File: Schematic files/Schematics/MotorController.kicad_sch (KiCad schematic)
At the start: 5 parts, among them M1 Z-Axis Stepper Motor

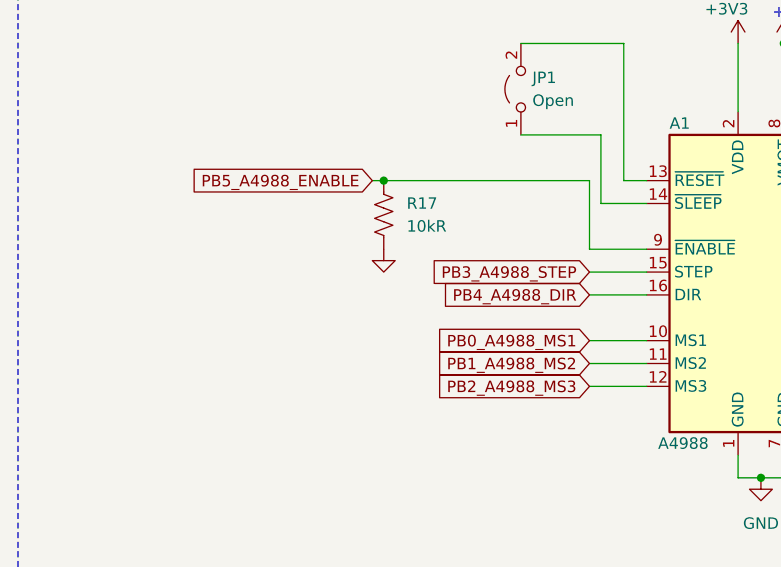
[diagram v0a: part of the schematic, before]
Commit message: pcb
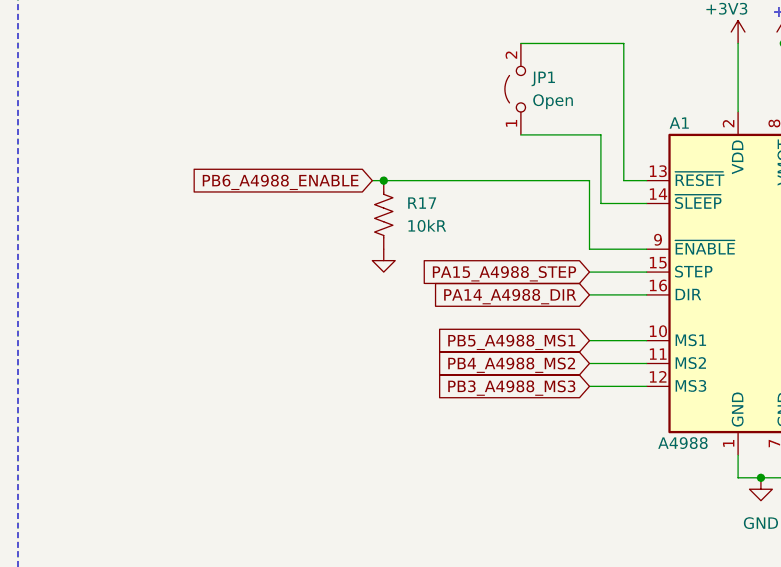
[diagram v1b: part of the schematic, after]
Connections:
- net PB0_A4988_MS1 renamed PB5_A4988_MS1
- net PB1_A4988_MS2 renamed PB4_A4988_MS2
- net PB2_A4988_MS3 renamed PB3_A4988_MS3
- net PB3_A4988_STEP renamed PA15_A4988_STEP
- net PB4_A4988_DIR renamed PA14_A4988_DIR
- net PB5_A4988_ENABLE renamed PB6_A4988_ENABLE
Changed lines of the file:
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@@
     (effects (font (size 1.27 1.27)) (justify left bottom))
   )
-  (global_label "PB1_A4988_MS2" (shape input) (at 115.57 73.66 180) (fields_autoplaced)
+  (global_label "PB4_A4988_MS2" (shape input) (at 115.57 73.66 180) (fields_autoplaced)
     (effects (font (size 1.27 1.27)) (justify right))
     (property "Intersheetrefs" "${INTERSHEET_REFS}" (at 97.1031 73.66 0)
@@
     )
   )
-  (global_label "PB5_A4988_ENABLE" (shape input) (at 91.44 53.34 180) (fields_autoplaced)
+  (global_label "PB6_A4988_ENABLE" (shape input) (at 91.44 53.34 180) (fields_autoplaced)
     (effects (font (size 1.27 1.27)) (justify right))
     (property "Intersheetrefs" "${INTERSHEET_REFS}" (at 69.8283 53.34 0)
@@
     )
   )
-  (global_label "PB0_A4988_MS1" (shape input) (at 115.57 71.12 180) (fields_autoplaced)
+  (global_label "PB5_A4988_MS1" (shape input) (at 115.57 71.12 180) (fields_autoplaced)
     (effects (font (size 1.27 1.27)) (justify right))
     (property "Intersheetrefs" "${INTERSHEET_REFS}" (at 97.1031 71.12 0)
@@
     )
   )
-  (global_label "PB2_A4988_MS3" (shape input) (at 115.57 76.2 180) (fields_autoplaced)
+  (global_label "PB3_A4988_MS3" (shape input) (at 115.57 76.2 180) (fields_autoplaced)
     (effects (font (size 1.27 1.27)) (justify right))
     (property "Intersheetrefs" "${INTERSHEET_REFS}" (at 97.1031 76.2 0)
@@
     )
   )
-  (global_label "PB3_A4988_STEP" (shape input) (at 115.57 63.5 180) (fields_autoplaced)
+  (global_label "PA15_A4988_STEP" (shape input) (at 115.57 63.5 180) (fields_autoplaced)
     (effects (font (size 1.27 1.27)) (justify right))
-    (property "Intersheetrefs" "${INTERSHEET_REFS}" (at 96.3774 63.5 0)
+    (property "Intersheetrefs" "${INTERSHEET_REFS}" (at 95.3493 63.5 0)
       (effects (font (size 1.27 1.27)) (justify right) hide)
     )
   )
-  (global_label "PB4_A4988_DIR" (shape input) (at 115.57 66.04 180) (fields_autoplaced)
+  (global_label "PA14_A4988_DIR" (shape input) (at 115.57 66.04 180) (fields_autoplaced)
     (effects (font (size 1.27 1.27)) (justify right))
-    (property "Intersheetrefs" "${INTERSHEET_REFS}" (at 97.8287 66.04 0)
+    (property "Intersheetrefs" "${INTERSHEET_REFS}" (at 96.8006 66.04 0)
       (effects (font (size 1.27 1.27)) (justify right) hide)
     )
